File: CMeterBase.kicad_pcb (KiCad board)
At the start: 2 copper layers, 74.4 x 103.6 mm, 24 parts, among them J1 Screw_Terminal_01x02, J2 PCB_CONN, Q1 Q_NPN_ECB, T1 L_Measure, T2 TPK-1-6

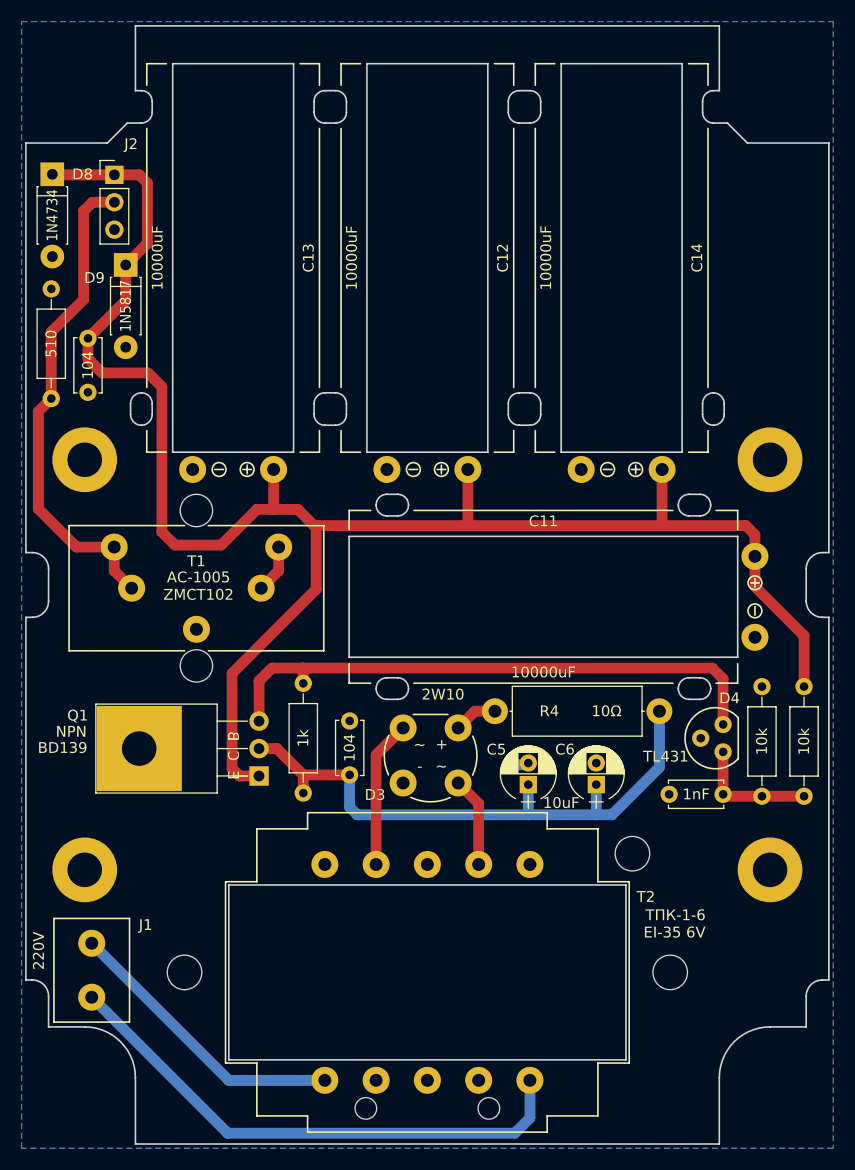
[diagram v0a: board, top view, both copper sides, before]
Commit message: update
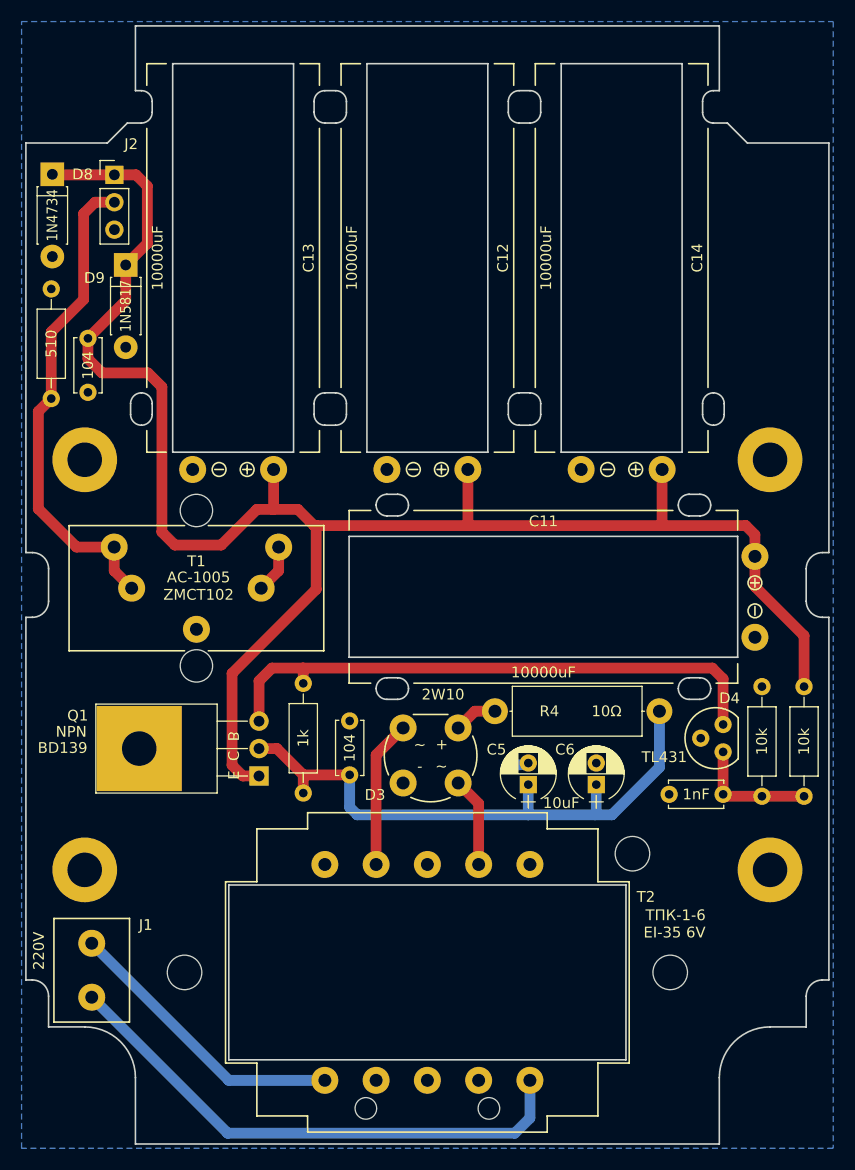
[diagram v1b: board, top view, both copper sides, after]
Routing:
- net +5V: track 165.6 -> 165.1 mm
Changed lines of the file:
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@@
     (thickness 1.6)
     (drawings 5)
-    (tracks 85)
+    (tracks 83)
     (zones 0)
     (modules 24)
@@
   )
   (setup
-    (last_trace_width 1)
+    (last_trace_width 0.5)
     (user_trace_width 0.5)
     (user_trace_width 0.8)
@@
     (visible_elements 7FFFFF7F)
     (pcbplotparams
-      (layerselection 0x00030_80000001)
+      (layerselection 0x010f0_80000001)
       (usegerberextensions false)
       (excludeedgelayer true)
@@
       (outputformat 1)
       (mirror false)
-      (drillshape 1)
+      (drillshape 0)
       (scaleselection 1)
-      (outputdirectory ""))
+      (outputdirectory GerberBase))
   )
   (net 0 "")
@@
       (effects (font (size 1 1) (thickness 0.15)))
     )
-    (fp_text value TL431 (at -1.7 -4.5 180) (layer F.Fab)
-      (effects (font (size 1 1) (thickness 0.15)))
-    )
-    (fp_text user TL431 (at -1.7 -4.5 180) (layer F.SilkS)
+    (fp_text value TL431 (at -1.75 -4.65 180) (layer F.Fab)
+      (effects (font (size 1 1) (thickness 0.15)))
+    )
+    (fp_text user TL431 (at -1.75 -4.65 180) (layer F.SilkS)
       (effects (font (size 1 1) (thickness 0.15)))
     )
@@
   (segment (start 86.22 96.49) (end 86.22 98.68) (width 1) (layer F.Cu) (net 2))
   (segment (start 86.22 98.68) (end 84.6 100.3) (width 1) (layer F.Cu) (net 2))
-  (segment (start 127.4 119.4) (end 127.58 119.58) (width 1) (layer F.Cu) (net 3))
   (segment (start 127.4 119.4) (end 127.4 115.47) (width 1) (layer F.Cu) (net 3))
   (segment (start 127.58 119.58) (end 131 119.58) (width 1) (layer F.Cu) (net 3))
@@
   (segment (start 71 62) (end 65.3 62) (width 1) (layer F.Cu) (net 4))
   (segment (start 72.05 70.35) (end 74.05 68.35) (width 1) (layer F.Cu) (net 4))
-  (segment (start 73.3 62) (end 71 62) (width 1) (layer F.Cu) (net 4))
-  (segment (start 74.05 62.75) (end 73.3 62) (width 1) (layer F.Cu) (net 4))
-  (segment (start 74.05 68.35) (end 74.05 62.75) (width 1) (layer F.Cu) (net 4))
+  (segment (start 73 62) (end 71 62) (width 1) (layer F.Cu) (net 4))
+  (segment (start 74.05 63.05) (end 73 62) (width 1) (layer F.Cu) (net 4))
+  (segment (start 74.05 68.35) (end 74.05 63.05) (width 1) (layer F.Cu) (net 4))
   (segment (start 75.4 81.65) (end 74.1 80.35) (width 1) (layer F.Cu) (net 4))
   (segment (start 75.4 95.1) (end 75.4 81.65) (width 1) (layer F.Cu) (net 4))
@@
   (segment (start 72.05 73.65) (end 72.05 70.35) (width 1) (layer F.Cu) (net 4))
   (segment (start 89.7 100.4) (end 89.7 94.5) (width 1) (layer F.Cu) (net 4))
-  (segment (start 82.6 117.7) (end 81.9 117) (width 1) (layer F.Cu) (net 4))
-  (segment (start 81.9 117) (end 81.9 108.2) (width 1) (layer F.Cu) (net 4))
+  (segment (start 82.9 117.7) (end 81.9 116.7) (width 1) (layer F.Cu) (net 4))
+  (segment (start 81.9 116.7) (end 81.9 108.2) (width 1) (layer F.Cu) (net 4))
   (segment (start 81.9 108.2) (end 89.7 100.4) (width 1) (layer F.Cu) (net 4))
-  (segment (start 84.4 117.7) (end 82.6 117.7) (width 1) (layer F.Cu) (net 4))
-  (segment (start 89.7 94.5) (end 89.5 94.5) (width 1) (layer F.Cu) (net 4))
+  (segment (start 84.4 117.7) (end 82.9 117.7) (width 1) (layer F.Cu) (net 4))
   (segment (start 85.75 89.3) (end 85.75 93) (width 1) (layer F.Cu) (net 4))
   (segment (start 103.75 94.5) (end 89.5 94.5) (width 1) (layer F.Cu) (net 4))
@@
   (segment (start 65.15 76.55) (end 68.15 73.55) (width 1) (layer F.Cu) (net 11))
   (segment (start 65.15 82.73) (end 65.15 76.55) (width 1) (layer F.Cu) (net 11))
-  (segment (start 68.96 64.54) (end 71 64.54) (width 1) (layer F.Cu) (net 11))
-  (segment (start 68.15 65.35) (end 68.96 64.54) (width 1) (layer F.Cu) (net 11))
-  (segment (start 68.15 73.55) (end 68.15 65.35) (width 1) (layer F.Cu) (net 11))
+  (segment (start 69.21 64.54) (end 71 64.54) (width 1) (layer F.Cu) (net 11))
+  (segment (start 68.15 65.6) (end 69.21 64.54) (width 1) (layer F.Cu) (net 11))
+  (segment (start 68.15 73.55) (end 68.15 65.6) (width 1) (layer F.Cu) (net 11))
   (segment (start 67.49 96.49) (end 63.95 92.95) (width 1) (layer F.Cu) (net 11))
   (segment (start 70.98 96.49) (end 67.49 96.49) (width 1) (layer F.Cu) (net 11))
